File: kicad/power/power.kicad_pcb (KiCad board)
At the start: 2 copper layers, 5 parts, among them J1 Power IN, J2 Power OUT, SW1 SW_SPST

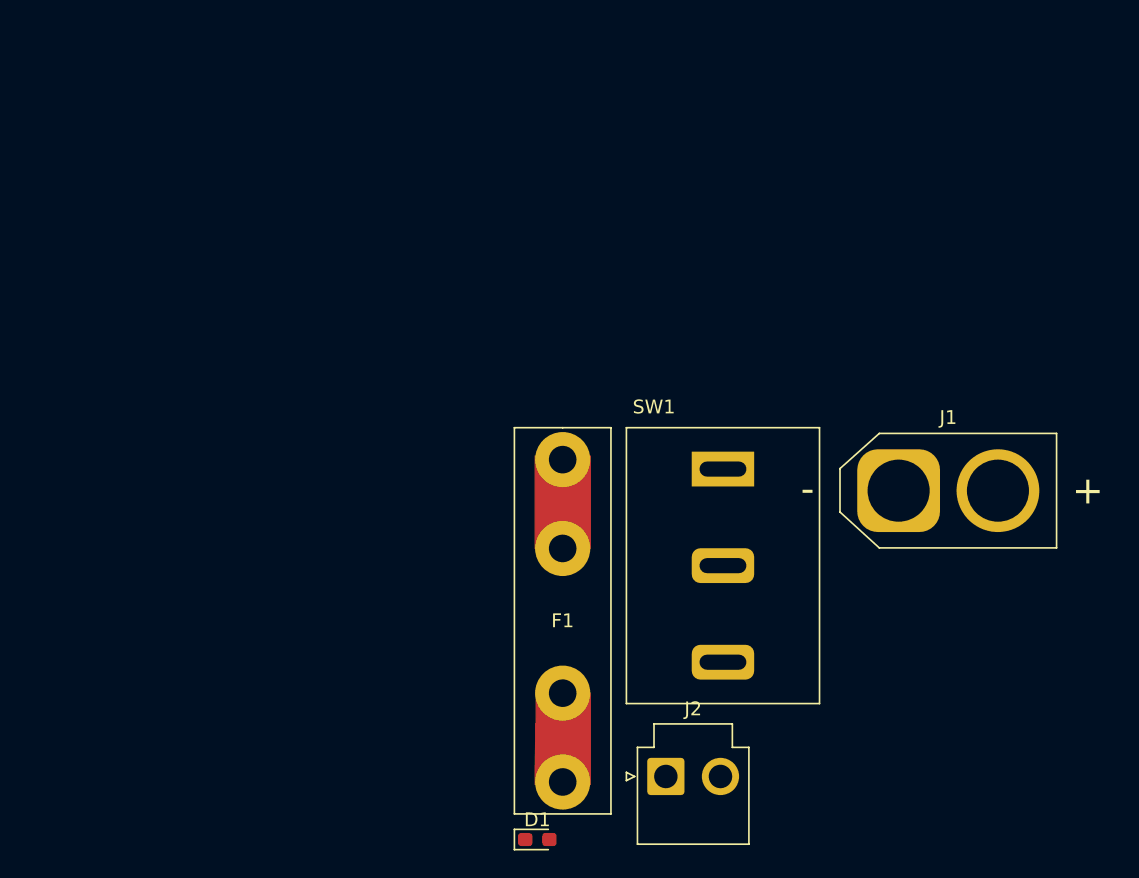
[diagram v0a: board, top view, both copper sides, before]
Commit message: power
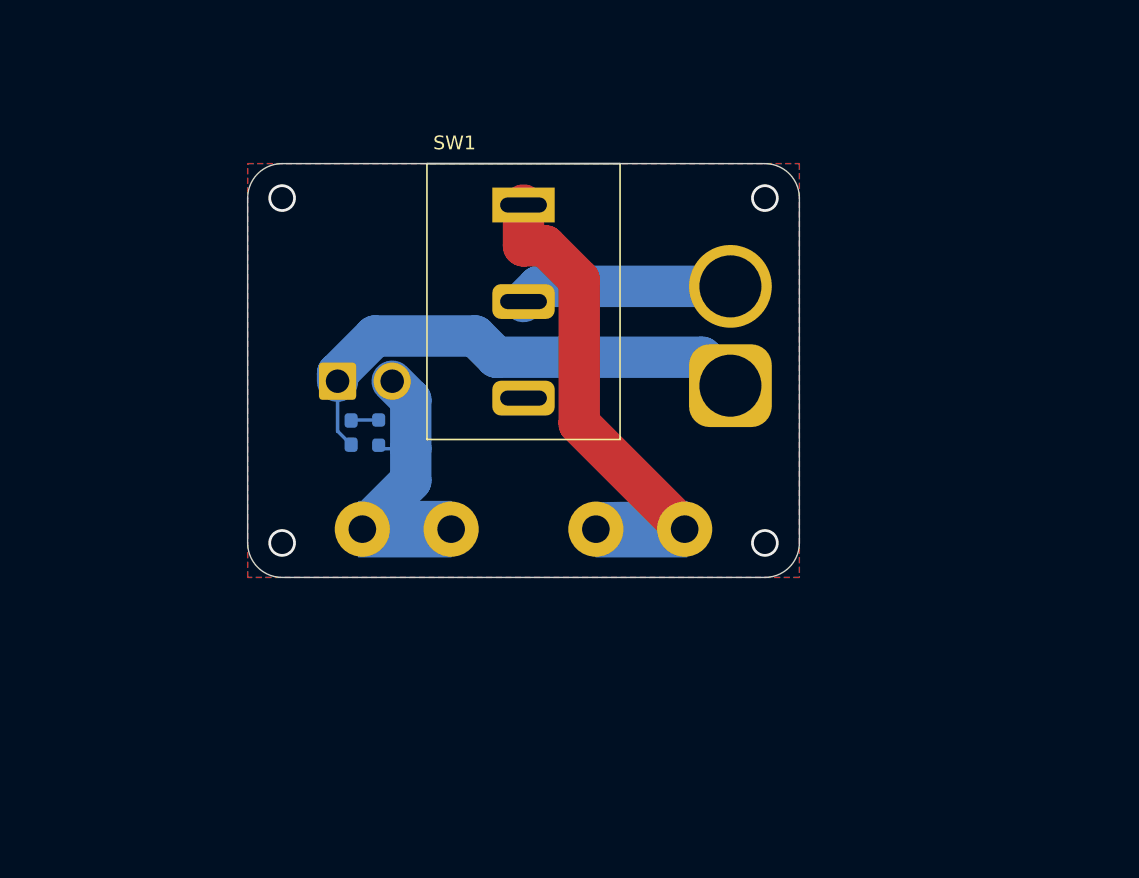
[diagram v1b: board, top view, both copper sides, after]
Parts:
- added R1: 3k, Resistor_SMD:R_0603_1608Metric_Pad0.98x0.95mm_HandSolder, B.Cu at (109.5, 89.5)
- D1, F1, J1: moved to B.Cu
- J2: footprint Connector_JST:JST_VH_B2P-VH-B_1x02_P3.96mm_Vertical -> Connector_JST:JST_VH_B2PS-VH_1x02_P3.96mm_Horizontal; moved to B.Cu
- moved J2 37.2 mm to (106.5, 85.8)
- moved D1 32.4 mm to (107.5, 89.5), turned to 90 degrees
- moved SW1 24.0 mm to (120.0, 80.0)
- moved J1 14.4 mm to (135.0, 86.1), turned to 90 degrees
- moved F1 7.23 mm to (120.0, 96.5), turned to -90 degrees
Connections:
- net Net-(D1-Pad1) renamed GND
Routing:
- net GND: track 0.00 -> 36.7 mm
- net Net-(F1-Pad2): track 0.00 -> 29.3 mm
- net Net-(J1-Pad2): track 0.00 -> 15.5 mm
- net Net-(F1-Pad1): track 0.00 -> 15.2 mm
- net Net-(D1-Pad2): track 0.00 -> 2.02 mm
- net (no net): vias 0 -> 4
- added copper zone on B.Cu, net GND
- added copper zone on F.Cu, net GND
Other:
- board outline added: 40 x 30 mm

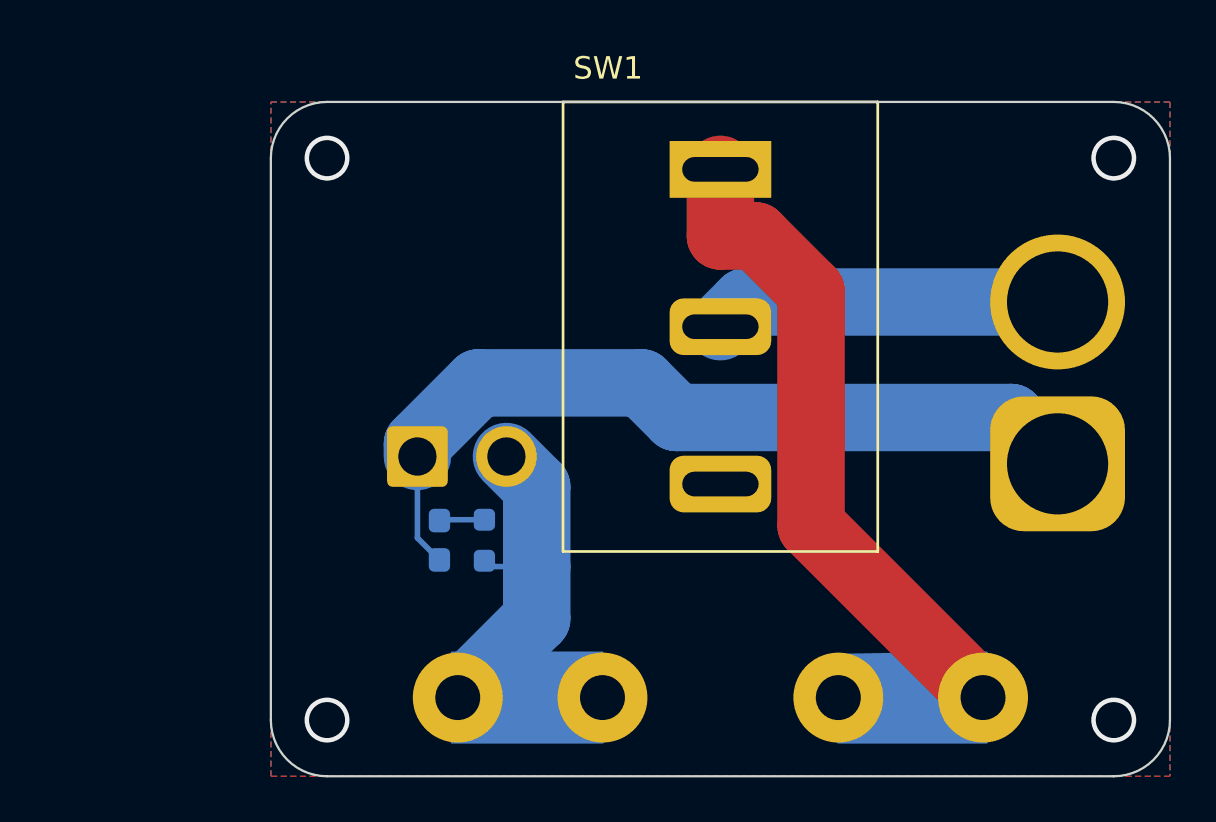
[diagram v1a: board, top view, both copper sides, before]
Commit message: no message
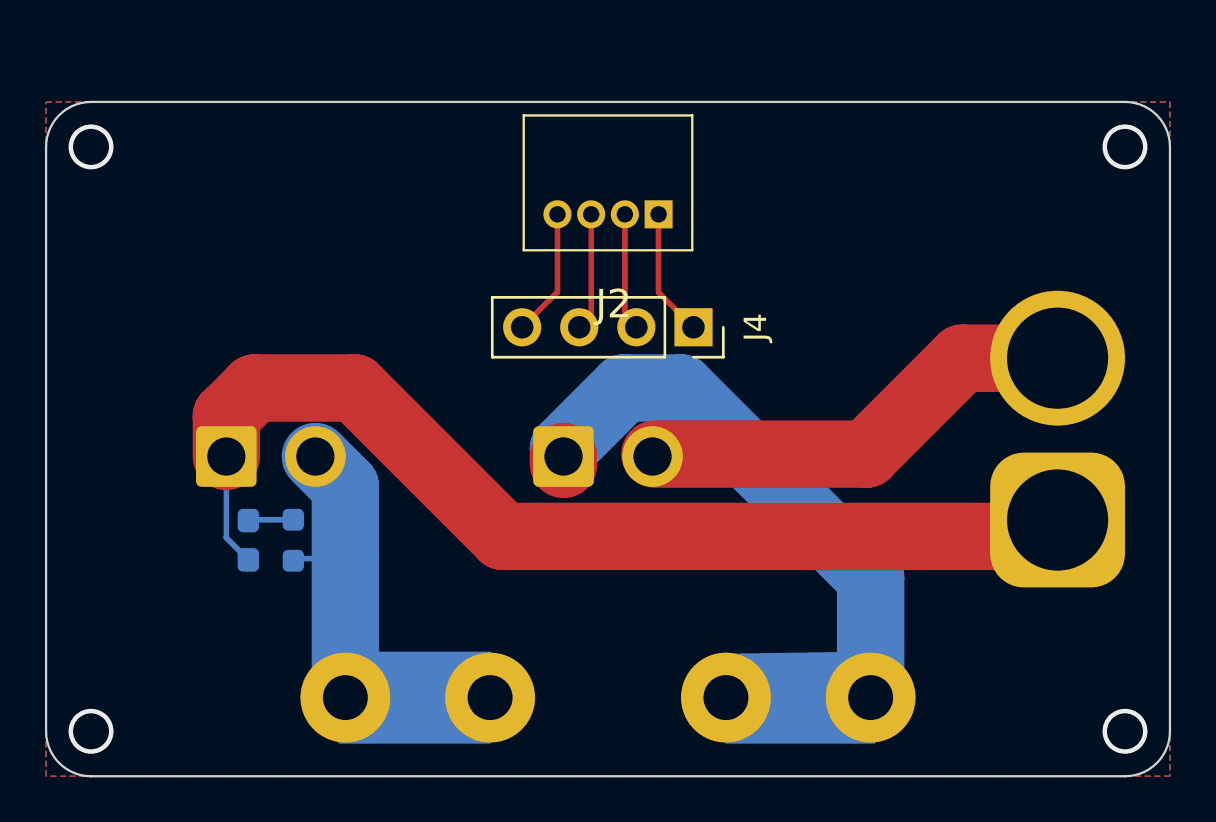
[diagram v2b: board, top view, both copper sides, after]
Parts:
- removed SW1: SW_SPST, 0.main.robot:SW_SPST_POWER
- added J2: OLED_in, 0.main.robot:JSTS4B-ZRLFSN, F.Cu at (115.0, 75.0)
- added J3: SW_Power, Connector_JST:JST_VH_B2PS-VH_1x02_P3.96mm_Horizontal, B.Cu at (113.0, 85.8)
- added J4: OLED_out, Connector_PinSocket_2.54mm:PinSocket_1x04_P2.54mm_Vertical, F.Cu at (118.8, 80.0)
- moved D1 8.50 mm to (99.0, 89.5)
- moved J5 8.50 mm to (98.0, 85.8)
- moved R1 8.50 mm to (101.0, 89.5)
- moved F1 5.00 mm to (115.0, 96.5)
- moved J1 2.50 mm to (135.0, 88.6)
- renumbered J2 to J5
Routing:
- net GND: track 36.7 -> 47.3 mm
- net Net-(J2-Pad4): track 0.00 -> 5.68 mm
- net Net-(J2-Pad1): track 0.00 -> 5.67 mm
- net Net-(J2-Pad3): track 0.00 -> 5.24 mm
- net Net-(J2-Pad2): track 0.00 -> 5.24 mm
- net Net-(F1-Pad2): track 29.3 -> 24.3 mm
- net Net-(J1-Pad2): track 15.5 -> 19.7 mm
- net Net-(F1-Pad1): track 15.2 -> 13.6 mm
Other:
- board size 40 x 30 mm -> 50 x 30 mm

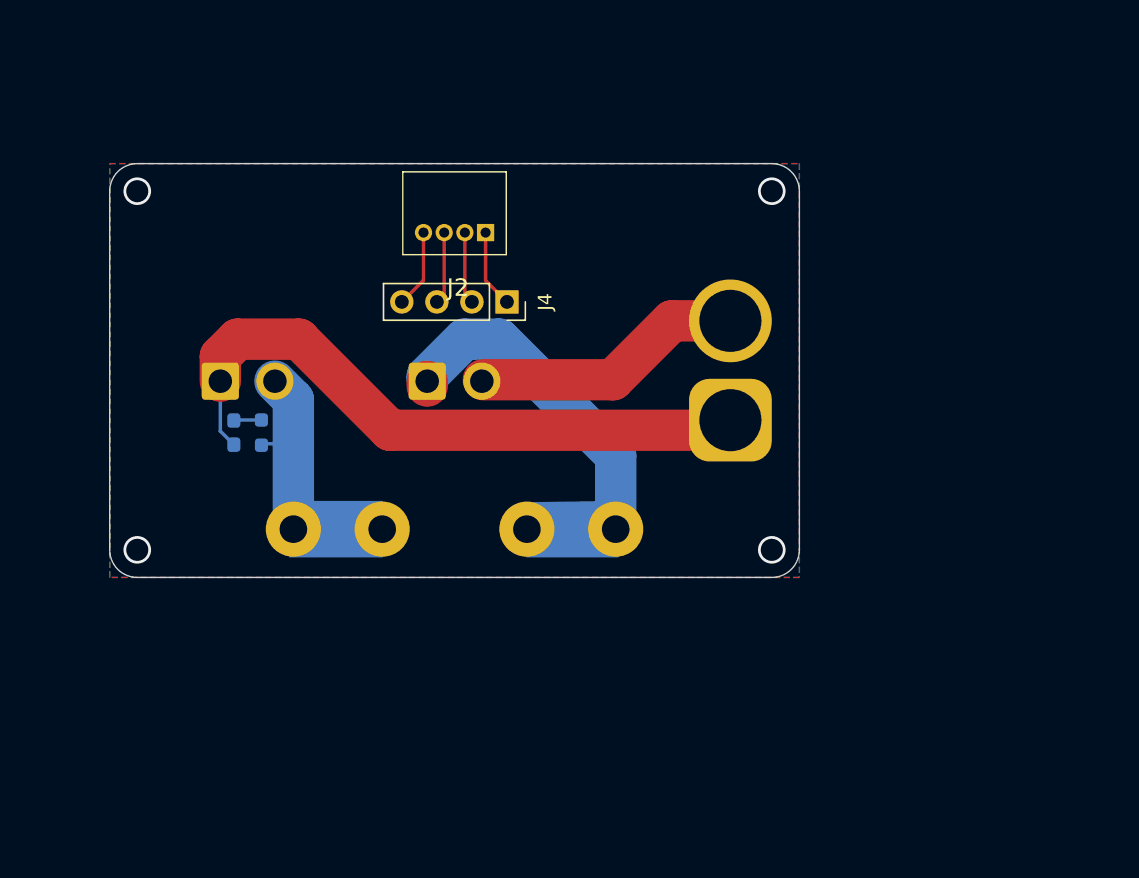
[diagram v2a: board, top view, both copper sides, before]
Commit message: fix: power
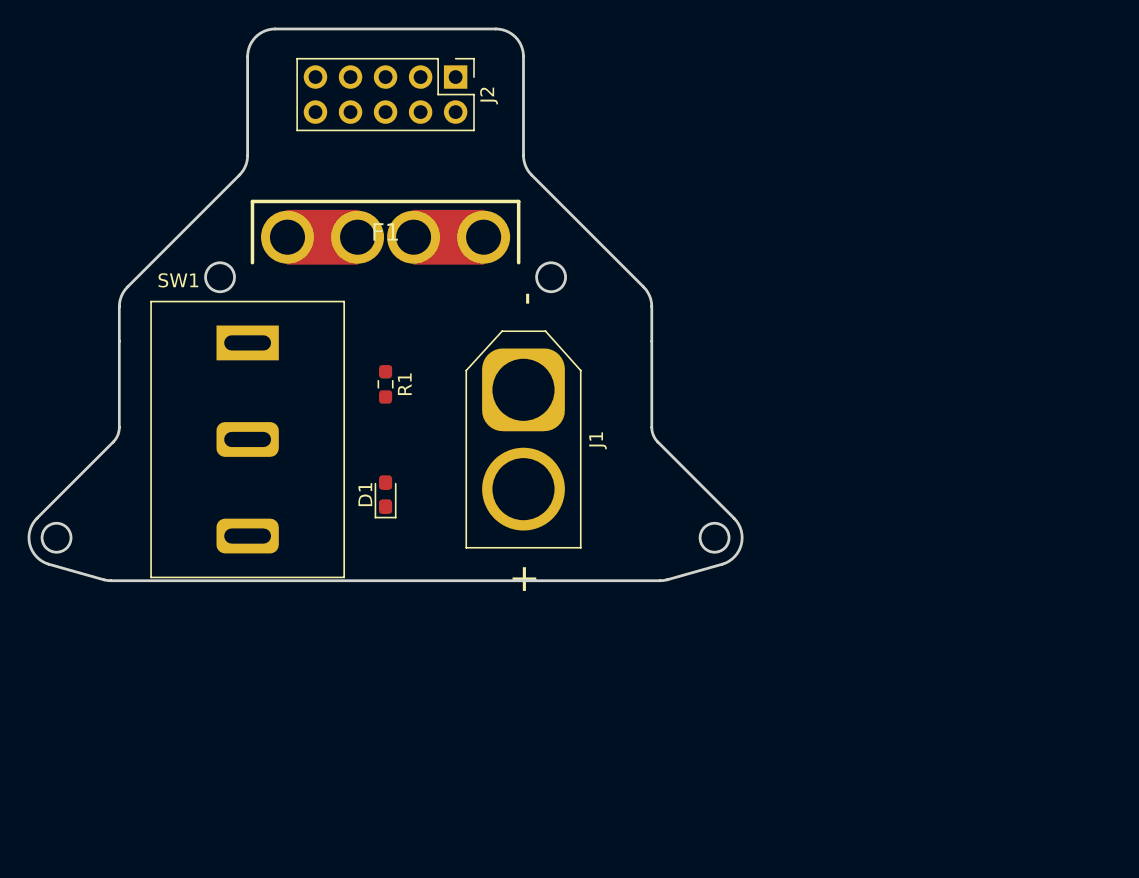
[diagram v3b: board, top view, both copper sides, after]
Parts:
- removed J3: SW_Power, Connector_JST:JST_VH_B2PS-VH_1x02_P3.96mm_Horizontal
- removed J4: OLED_out, Connector_PinSocket_2.54mm:PinSocket_1x04_P2.54mm_Vertical
- removed J5: Power OUT, Connector_JST:JST_VH_B2PS-VH_1x02_P3.96mm_Horizontal
- added SW1: SW_SPST, 0.main.robot:SW_SPST_POWER, F.Cu at (100.0, 90.0)
- D1, J1, R1: moved to F.Cu
- F1: footprint 0.main.robot:FUSE_20mm -> 0.main.robot:FUSE_35222; moved to F.Cu
- J2: value OLED_in -> Power OUT; footprint 0.main.robot:JSTS4B-ZRLFSN -> Connector_PinHeader_2.54mm:PinHeader_2x05_P2.54mm_Vertical
- moved F1 20.0 mm to (110.0, 77.2), turned to 180 degrees
- moved J1 15.2 mm to (120.0, 86.4), turned to -90 degrees
- moved D1 11.9 mm to (110.0, 94.0)
- moved J2 11.3 mm to (115.1, 63.7), turned to -90 degrees
- moved R1 9.66 mm to (110.0, 86.0), turned to -90 degrees
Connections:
- J2 pad 1: Net-(J2-Pad1) -> GND
- J2 pad 2: Net-(J2-Pad2) -> Net-(F1-Pad1)
- J2 pad 3: Net-(J2-Pad3) -> GND
- J2 pad 4: Net-(J2-Pad4) -> Net-(F1-Pad1)
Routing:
- net GND: track 47.3 -> 0.00 mm
- net Net-(F1-Pad2): track 24.3 -> 0.00 mm
- net Net-(J1-Pad2): track 19.7 -> 0.00 mm
- net Net-(F1-Pad1): track 13.6 -> 0.00 mm
- net Net-(J2-Pad4): track 5.68 -> 0.00 mm
- net Net-(J2-Pad1): track 5.67 -> 0.00 mm
- net Net-(J2-Pad3): track 5.24 -> 0.00 mm
- net Net-(J2-Pad2): track 5.24 -> 0.00 mm
- net Net-(D1-Pad2): track 2.02 -> 0.00 mm
- net (no net): vias 4 -> 0
- removed copper zone on B.Cu, net GND
- removed copper zone on F.Cu, net GND
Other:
- board size 50 x 30 mm -> 51.7 x 40 mm
